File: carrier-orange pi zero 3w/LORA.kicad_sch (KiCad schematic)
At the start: 2 parts, among them J15 LORA_ANTENNA, J2 CORE1262_HF

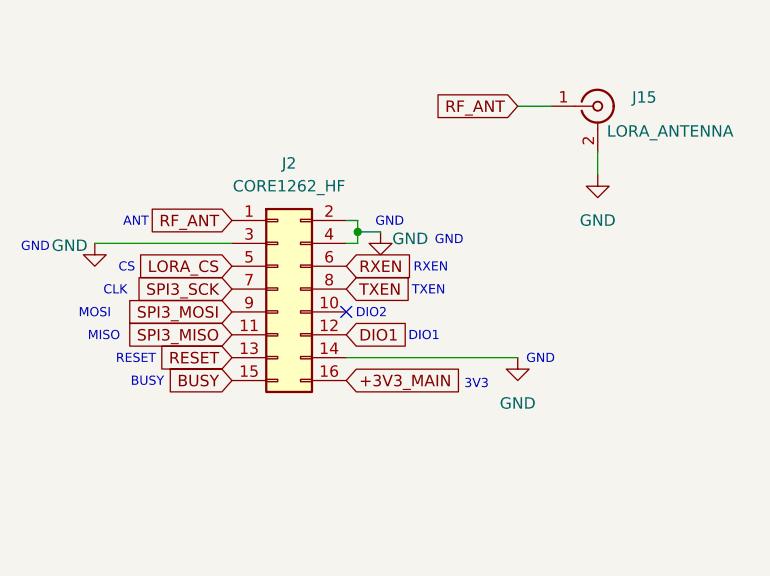
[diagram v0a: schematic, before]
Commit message: ain
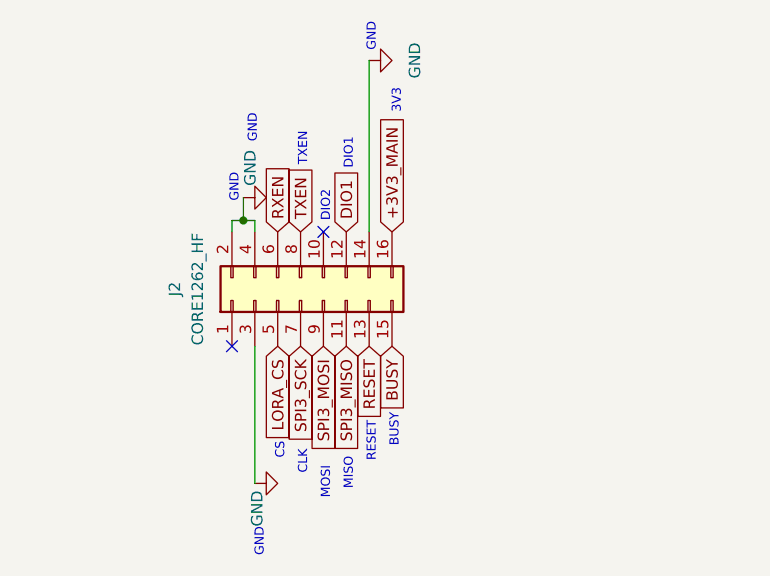
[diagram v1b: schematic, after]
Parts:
- removed J15: LORA_ANTENNA, symbol Connector:Conn_Coaxial
- J2: footprint (none) -> Waveshare_Core1262:Core1262_HF
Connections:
- net RF_ANT: no longer names the net of J2.1 (Pin_1)
- no-connect marks 1 -> 2
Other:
- note removed: "ANT"
- note removed: "RXEN"
- moved on the sheet: J2

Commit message: ain
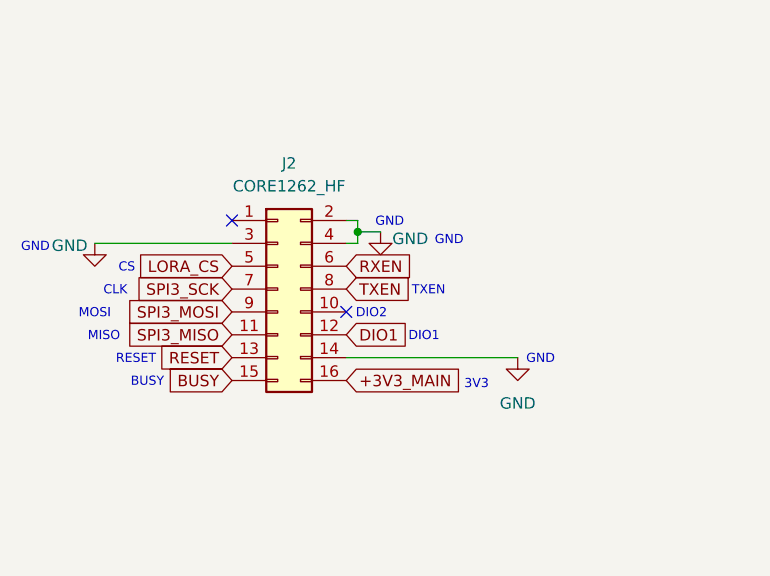
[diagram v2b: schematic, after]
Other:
- moved on the sheet: J2
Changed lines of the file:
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@@
 	(text "GND"
 		(exclude_from_sim no)
-		(at 110.744 43.18 90)
+		(at 129.54 78.994 0)
 		(effects
 			(font
@@
 	(text "DIO2"
 		(exclude_from_sim no)
-		(at 105.664 61.976 90)
+		(at 110.744 73.914 0)
 		(effects
 			(font
@@
 	(text "BUSY"
 		(exclude_from_sim no)
-		(at 113.284 86.868 90)
+		(at 85.852 81.534 0)
 		(effects
 			(font
@@
 	(text "GND"
 		(exclude_from_sim no)
-		(at 95.504 59.944 90)
+		(at 112.776 63.754 0)
 		(effects
 			(font
@@
 	(text "3V3"
 		(exclude_from_sim no)
-		(at 113.538 50.292 90)
+		(at 122.428 81.788 0)
 		(effects
 			(font
@@
 	(text "DIO1"
 		(exclude_from_sim no)
-		(at 108.204 56.134 90)
+		(at 116.586 76.454 0)
 		(effects
 			(font
@@
 	(text "GND"
 		(exclude_from_sim no)
-		(at 98.298 99.314 90)
+		(at 73.406 66.548 0)
 		(effects
 			(font
@@
 	(text "TXEN"
 		(exclude_from_sim no)
-		(at 103.124 55.626 90)
+		(at 117.094 71.374 0)
 		(effects
 			(font
@@
 	(text "GND"
 		(exclude_from_sim no)
-		(at 97.536 53.34 90)
+		(at 119.38 65.786 0)
 		(effects
 			(font
@@
 	(text "CLK"
 		(exclude_from_sim no)
-		(at 103.124 90.424 90)
+		(at 82.296 71.374 0)
 		(effects
 			(font
@@
 	(text "MOSI"
 		(exclude_from_sim no)
-		(at 105.664 92.71 90)
+		(at 80.01 73.914 0)
 		(effects
 			(font
@@
 	(text "MISO"
 		(exclude_from_sim no)
-		(at 108.204 91.694 90)
+		(at 81.026 76.454 0)
 		(effects
 			(font
@@
 	(text "RESET"
 		(exclude_from_sim no)
-		(at 110.744 88.138 90)
+		(at 84.582 78.994 0)
 		(effects
 			(font
@@
 	(text "CS"
 		(exclude_from_sim no)
-		(at 100.584 89.154 90)
+		(at 83.566 68.834 0)
 		(effects
 			(font
@@
 	)
 	(junction
-		(at 96.52 63.5)
+		(at 109.22 64.77)
 		(diameter 0)
 		(color 0 0 0 0)
 	)
 	(no_connect
-		(at 105.41 64.77)
+		(at 107.95 73.66)
 	)
 	(no_connect
-		(at 95.25 77.47)
+		(at 95.25 63.5)
 	)
 	(wire
 		(pts
-			(xy 97.79 92.71) (xy 97.79 77.47)
+			(xy 80.01 66.04) (xy 95.25 66.04)
 		)
 		(stroke
@@
 	(wire
 		(pts
-			(xy 110.49 64.77) (xy 110.49 45.72)
+			(xy 107.95 78.74) (xy 127 78.74)
 		)
 		(stroke
@@
 	(wire
 		(pts
-			(xy 97.79 63.5) (xy 97.79 64.77)
+			(xy 109.22 66.04) (xy 107.95 66.04)
 		)
 		(stroke
@@
 	(wire
 		(pts
-			(xy 95.25 63.5) (xy 96.52 63.5)
+			(xy 109.22 63.5) (xy 109.22 64.77)
 		)
 		(stroke
@@
 	(wire
 		(pts
-			(xy 96.52 63.5) (xy 97.79 63.5)
+			(xy 109.22 64.77) (xy 109.22 66.04)
 		)
 		(stroke
@@
 	(wire
 		(pts
-			(xy 95.25 64.77) (xy 95.25 63.5)
+			(xy 107.95 63.5) (xy 109.22 63.5)
 		)
 		(stroke
@@
 	(wire
 		(pts
-			(xy 96.52 63.5) (xy 96.52 60.96)
+			(xy 109.22 64.77) (xy 111.76 64.77)
 		)
 		(stroke
@@
 	(global_label "SPI3_MOSI "
 		(shape input)
-		(at 105.41 77.47 270)
+		(at 95.25 73.66 180)
 		(fields_autoplaced yes)
 		(effects
@@
 		)
 		(property "Intersheetrefs" "${INTERSHEET_REFS}"
-			(at 105.41 91.2804 90)
+			(at 81.4396 73.66 0)
 			(hide yes)
 			(show_name no)
@@
 	(global_label "+3V3_MAIN"
 		(shape input)
-		(at 113.03 64.77 90)
+		(at 107.95 81.28 0)
 		(fields_autoplaced yes)
 		(effects
@@
 		)
 		(property "Intersheetrefs" "${INTERSHEET_REFS}"
-			(at 113.03 51.2619 90)
+			(at 121.4581 81.28 0)
 			(hide yes)
 			(show_name no)
@@
 	(global_label "TXEN"
 		(shape input)
-		(at 102.87 64.77 90)
+		(at 107.95 71.12 0)
 		(fields_autoplaced yes)
 		(effects
@@
 		)
 		(property "Intersheetrefs" "${INTERSHEET_REFS}"
-			(at 102.87 57.1282 90)
+			(at 115.5918 71.12 0)
 			(hide yes)
 			(show_name no)
@@
 	(global_label "SPI3_SCK"
 		(shape input)
-		(at 102.87 77.47 270)
+		(at 95.25 71.12 180)
 		(fields_autoplaced yes)
 		(effects
@@
 		)
 		(property "Intersheetrefs" "${INTERSHEET_REFS}"
-			(at 102.87 89.4661 90)
+			(at 83.2539 71.12 0)
 			(hide yes)
 			(show_name no)
@@
 	(global_label "RXEN"
 		(shape input)
-		(at 100.33 64.77 90)
+		(at 107.95 68.58 0)
 		(fields_autoplaced yes)
 		(effects
@@
 		)
 		(property "Intersheetrefs" "${INTERSHEET_REFS}"
-			(at 100.33 56.8258 90)
+			(at 115.8942 68.58 0)
 			(hide yes)
 			(show_name no)
@@
 	(global_label "DIO1"
 		(shape input)
-		(at 107.95 64.77 90)
+		(at 107.95 76.2 0)
 		(fields_autoplaced yes)
 		(effects
@@
 		)
 		(property "Intersheetrefs" "${INTERSHEET_REFS}"
-			(at 107.95 57.37 90)
+			(at 115.35 76.2 0)
 			(hide yes)
 			(show_name no)
@@
 	(global_label "BUSY"
 		(shape input)
-		(at 113.03 77.47 270)
+		(at 95.25 81.28 180)
 		(fields_autoplaced yes)
 		(effects
@@
 		)
 		(property "Intersheetrefs" "${INTERSHEET_REFS}"
-			(at 113.03 85.3538 90)
+			(at 87.3662 81.28 0)
 			(hide yes)
 			(show_name no)
@@
 	(global_label "SPI3_MISO"
 		(shape input)
-		(at 107.95 77.47 270)
+		(at 95.25 76.2 180)
 		(fields_autoplaced yes)
 		(effects
@@
 		)
 		(property "Intersheetrefs" "${INTERSHEET_REFS}"
-			(at 107.95 90.3128 90)
+			(at 82.4072 76.2 0)
 			(hide yes)
 			(show_name no)
@@
 	(global_label "LORA_CS"
 		(shape input)
-		(at 100.33 77.47 270)
+		(at 95.25 68.58 180)
 		(fields_autoplaced yes)
 		(effects
@@
 		)
 		(property "Intersheetrefs" "${INTERSHEET_REFS}"
-			(at 100.33 88.6195 90)
+			(at 84.1005 68.58 0)
 			(hide yes)
 			(show_name no)
@@
 	(global_label "RESET"
 		(shape input)
-		(at 110.49 77.47 270)
+		(at 95.25 78.74 180)
 		(fields_autoplaced yes)
 		(effects
@@
 		)
 		(property "Intersheetrefs" "${INTERSHEET_REFS}"
-			(at 110.49 86.2003 90)
+			(at 86.5197 78.74 0)
 			(hide yes)
 			(show_name no)
@@
 	(symbol
 		(lib_id "power:GND")
-		(at 96.52 60.96 90)
+		(at 111.76 64.77 0)
 		(unit 1)
 		(body_style 1)
@@
 		(dnp no)
 		(property "Reference" "#PWR013"
-			(at 102.87 60.96 0)
+			(at 111.76 71.12 0)
 			(hide yes)
 			(show_name no)
@@
 		)
 		(property "Value" "GND"
-			(at 97.282 57.658 0)
+			(at 115.062 65.532 0)
 			(show_name no)
 			(do_not_autoplace no)
@@
 		)
 		(property "Footprint" ""
-			(at 96.52 60.96 0)
+			(at 111.76 64.77 0)
 			(hide yes)
 			(show_name no)
@@
 		)
 		(property "Datasheet" ""
-			(at 96.52 60.96 0)
+			(at 111.76 64.77 0)
 			(hide yes)
 			(show_name no)
@@
 		)
 		(property "Description" "Power symbol creates a global label with name \"GND\" , ground"
-			(at 96.52 60.96 0)
+			(at 111.76 64.77 0)
 			(hide yes)
 			(show_name no)
@@
 	(symbol
 		(lib_id "power:GND")
-		(at 97.79 92.71 90)
+		(at 80.01 66.04 0)
 		(unit 1)
 		(body_style 1)
@@
 		(dnp no)
 		(property "Reference" "#PWR012"
-			(at 104.14 92.71 0)
+			(at 80.01 72.39 0)
 			(hide yes)
 			(show_name no)
@@
 		)
 		(property "Value" "GND"
-			(at 98.044 95.504 0)
+			(at 77.216 66.294 0)
 			(show_name no)
 			(do_not_autoplace no)
@@
 		)
 		(property "Footprint" ""
-			(at 97.79 92.71 0)
+			(at 80.01 66.04 0)
 			(hide yes)
 			(show_name no)
@@
 		)
 		(property "Datasheet" ""
-			(at 97.79 92.71 0)
+			(at 80.01 66.04 0)
 			(hide yes)
 			(show_name no)
@@
 		)
 		(property "Description" "Power symbol creates a global label with name \"GND\" , ground"
-			(at 97.79 92.71 0)
+			(at 80.01 66.04 0)
 			(hide yes)
 			(show_name no)
@@
 	(symbol
 		(lib_id "Connector_Generic:Conn_02x08_Odd_Even")
-		(at 102.87 72.39 90)
+		(at 100.33 71.12 0)
 		(unit 1)
 		(body_style 1)
@@
 		(fields_autoplaced yes)
 		(property "Reference" "J2"
-			(at 88.9 71.12 0)
+			(at 101.6 57.15 0)
 			(show_name no)
 			(do_not_autoplace no)
@@
 		)
 		(property "Value" "CORE1262_HF"
-			(at 91.44 71.12 0)
+			(at 101.6 59.69 0)
 			(show_name no)
 			(do_not_autoplace no)
@@
 		)
 		(property "Footprint" "Waveshare_Core1262:Core1262_HF"
-			(at 102.87 72.39 0)
+			(at 100.33 71.12 0)
 			(hide yes)
 			(show_name no)
@@
 		)
 		(property "Datasheet" ""
-			(at 102.87 72.39 0)
+			(at 100.33 71.12 0)
 			(hide yes)
 			(show_name no)
@@
 		)
 		(property "Description" "Generic connector, double row, 02x08, odd/even pin numbering scheme (row 1 odd numbers, row 2 even numbers), script generated (kicad-library-utils/schlib/autogen/connector/)"
-			(at 102.87 72.39 0)
+			(at 100.33 71.12 0)
 			(hide yes)
 			(show_name no)
@@
 	(symbol
 		(lib_id "power:GND")
-		(at 110.49 45.72 90)
+		(at 127 78.74 0)
 		(unit 1)
 		(body_style 1)
@@
 		(fields_autoplaced yes)
 		(property "Reference" "#PWR014"
-			(at 116.84 45.72 0)
+			(at 127 85.09 0)
 			(hide yes)
 			(show_name no)
@@
 		)
 		(property "Value" "GND"
-			(at 115.57 45.72 0)
+			(at 127 83.82 0)
 			(show_name no)
 			(do_not_autoplace no)
@@
 		)
 		(property "Footprint" ""
-			(at 110.49 45.72 0)
+			(at 127 78.74 0)
 			(hide yes)
 			(show_name no)
@@
 		)
 		(property "Datasheet" ""
-			(at 110.49 45.72 0)
+			(at 127 78.74 0)
 			(hide yes)
 			(show_name no)
@@
 		)
 		(property "Description" "Power symbol creates a global label with name \"GND\" , ground"
-			(at 110.49 45.72 0)
-			(hide yes)
-			(show_name no)
+			(at 127 78.74 0)
+			(hide yes)
+			(show_name no)
